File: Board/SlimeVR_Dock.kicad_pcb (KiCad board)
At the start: 2 copper layers, 83.8 x 76.8 mm, 91 parts, among them J1_Control1 Conn_01x03_Pin, J1_MainPW1 USB_C_Receptacle_USB2.0_16P, J1_Monitor1 Conn_01x03_Pin, J1_Prog1 Conn_01x03_Pin, J2 USB_C_Receptacle_USB2.0_16P, J3 USB_C_Receptacle_USB2.0_16P, J4 USB_C_Receptacle_USB2.0_16P, J5 USB_C_Receptacle_USB2.0_16P, J6 USB_C_Receptacle_USB2.0_16P, J7 USB_C_Receptacle_USB2.0_16P, J8 USB_C_Receptacle_USB2.0_16P, J9 USB_C_Receptacle_USB2.0_16P, Q1 AO3401A, Q2 BC857, Q3 BC857, Q4 BC857, Q5 BC857, U1 ESP32-C3-WROOM-02, U10 INA226, U11 AP22652W6-7, U12 INA226, U13 INA226, U14 AP22652W6-7, U15 INA226, U16 INA226, U17 74HC165, U18 74HC165, U19 74HC595, U2 CH224K, U3 XC6220B331MR, U5 AP22652W6-7, U6 INA226, U7 INA226, U8 AP22652W6-7, U9 INA226

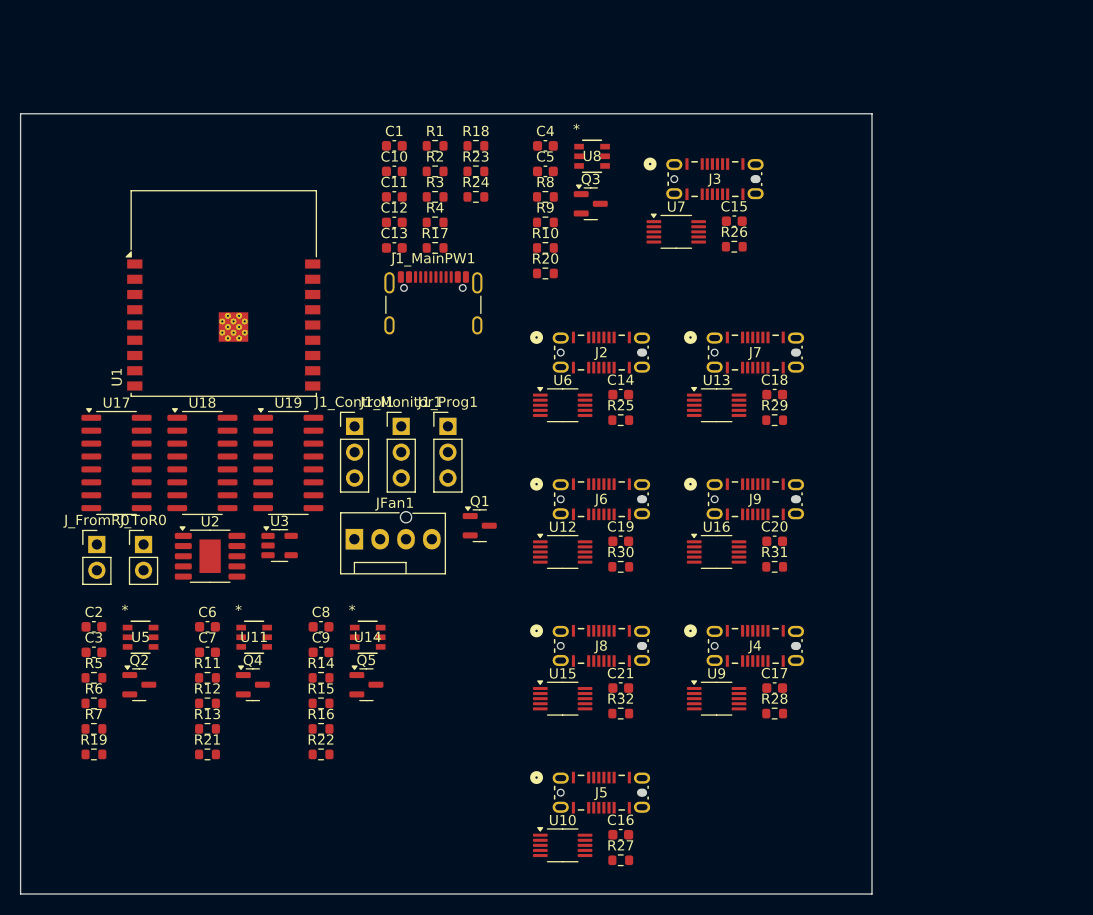
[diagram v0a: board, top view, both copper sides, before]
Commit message: Updavení USB-C
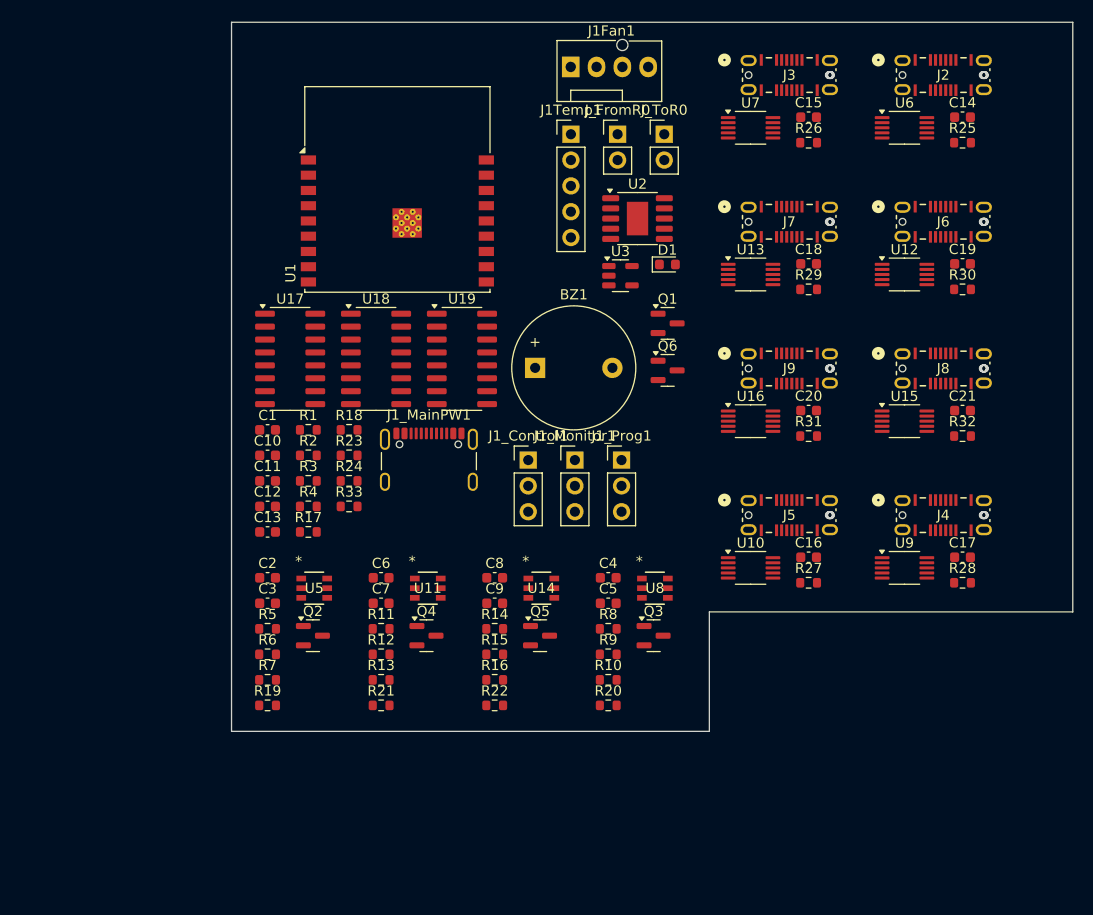
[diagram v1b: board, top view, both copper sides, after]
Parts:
- removed JFan1: Conn_01x04_Pin, Connector:FanPinHeader_1x04_P2.54mm_Vertical
- added BZ1: Buzzer, Buzzer_Beeper:Buzzer_12x9.5RM7.6, F.Cu at (121.4, 72.0)
- added D1: 1N4148, Diode_SMD:D_0603_1608Metric, F.Cu at (134.4, 61.8)
- added J1Fan1: Conn_01x04_Pin, Connector:FanPinHeader_1x04_P2.54mm_Vertical, F.Cu at (124.9, 42.4)
- added J1Temp1: Conn_01x05_Pin, Connector_PinHeader_2.54mm:PinHeader_1x05_P2.54mm_Vertical, F.Cu at (124.9, 49.0)
- added Q6: BC817, Package_TO_SOT_SMD:SOT-23, F.Cu at (134.4, 72.2)
- added R33: 1k, Resistor_SMD:R_0603_1608Metric, F.Cu at (103.1, 85.6)
- moved J_FromR0 65.2 mm to (129.5, 49.0)
- moved J_ToR0 65.2 mm to (134.1, 49.0)
- moved U2 53.6 mm to (131.4, 57.3)
- moved C19 43.3 mm to (163.4, 61.8)
- moved R32 43.3 mm to (163.4, 78.7)
- moved C14 43.3 mm to (163.4, 47.3)
- moved C21 43.3 mm to (163.4, 76.2)
- moved J2 43.3 mm to (161.5, 43.2)
- moved J6 43.3 mm to (161.5, 57.6)
- moved R25 43.3 mm to (163.4, 49.8)
- moved R30 43.3 mm to (163.4, 64.3)
- moved U12 43.3 mm to (157.7, 62.8)
- moved U6 43.3 mm to (157.7, 48.4)
- moved J8 43.3 mm to (161.5, 72.1)
- moved U15 43.3 mm to (157.7, 77.2)
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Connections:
- U19 pad 4: unconnected-(U19-QE-Pad4) -> BZ
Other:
- board size 83.8 x 76.8 mm -> 82.8 x 69.8 mm
